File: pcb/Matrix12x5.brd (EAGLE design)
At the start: 68 parts, among them IC1 4017D

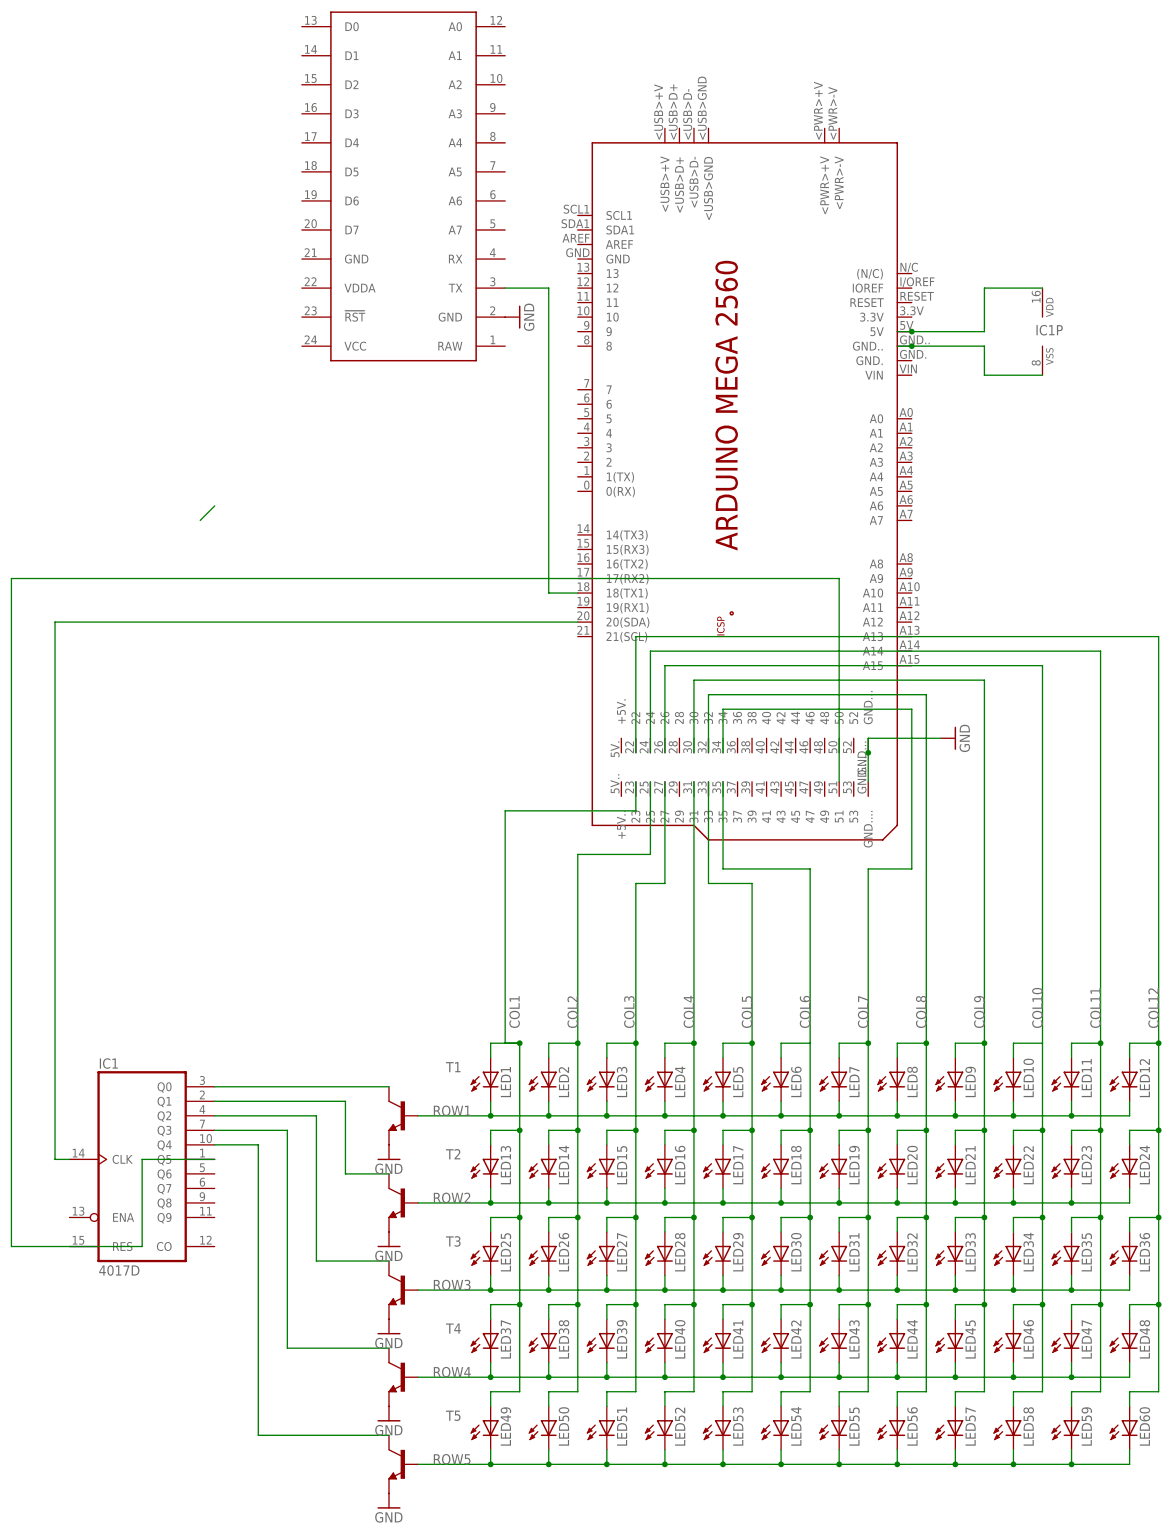
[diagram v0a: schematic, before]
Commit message: Cleanup in schematic
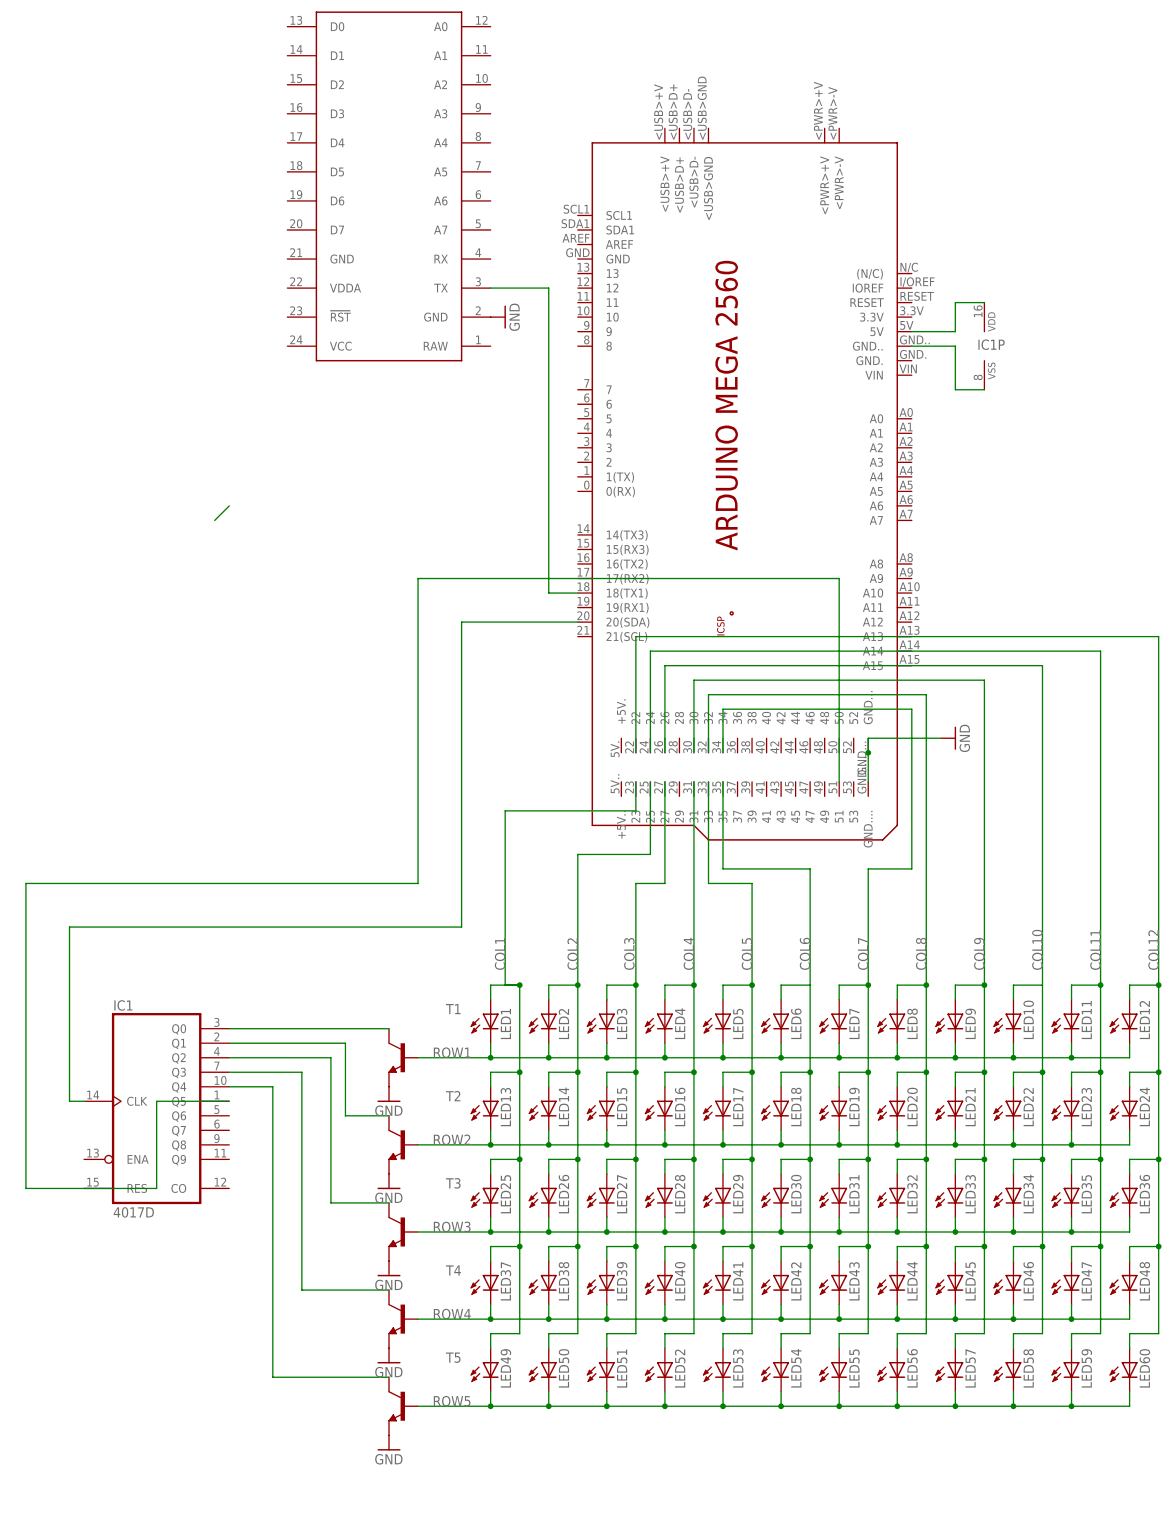
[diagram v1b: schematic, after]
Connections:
- new net N$12: IC1A.Q5, IC1A.RES
- net N$8: no longer IC1A.Q5, IC1A.RES
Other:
- moved on the sheet: IC1, IC1P, LED1, LED10, LED11, LED12, LED13, LED14, LED15, LED16, LED17, LED18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
